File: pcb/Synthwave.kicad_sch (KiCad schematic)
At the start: 61 parts, among them J1 Conn_01x01_Pin, J2 Conn_01x01_Pin, P1 MINI-360, P2 MINI-360, Q1 TIP120, Q10 TIP120, Q2 TIP120, Q3 TIP120, Q4 TIP120, Q5 TIP120, Q6 TIP120, Q7 TIP120, Q8 TIP120, Q9 TIP120, U1 Heltec_HTIT-WB32, U2 L9110

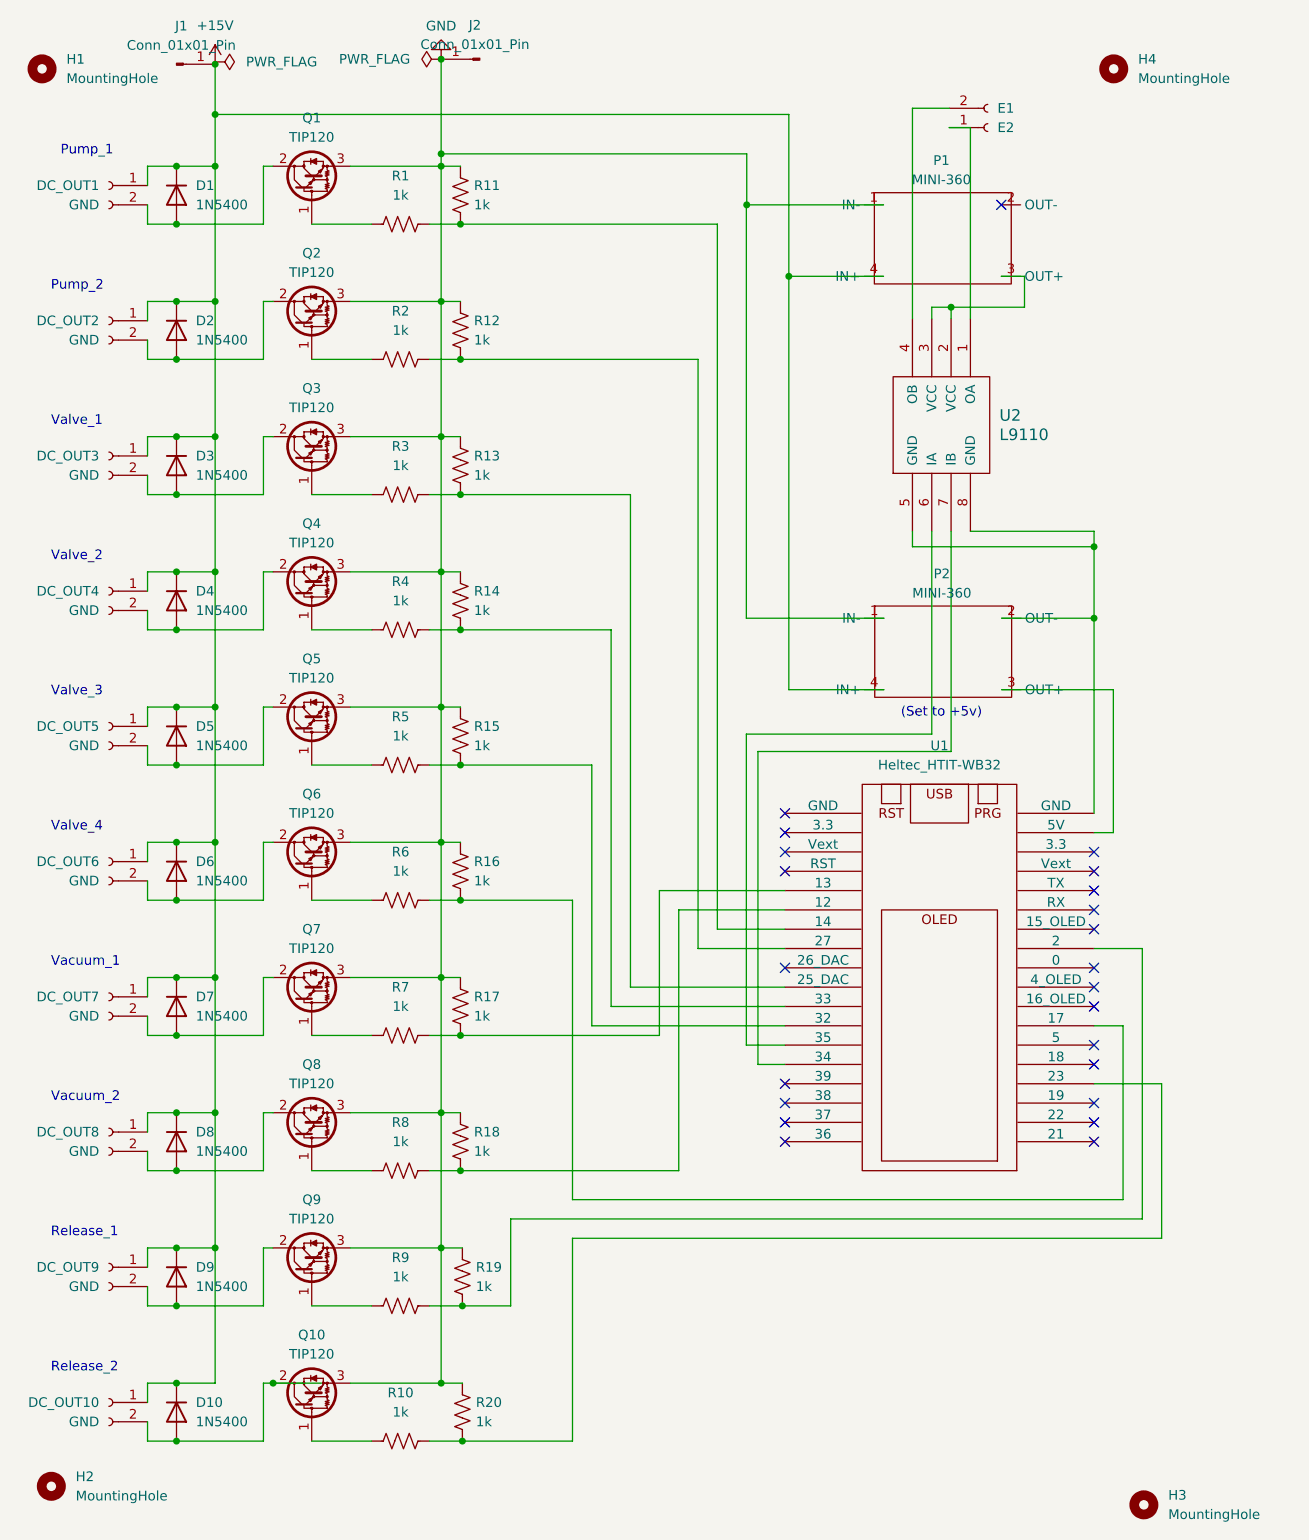
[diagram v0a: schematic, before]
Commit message: Many small updates
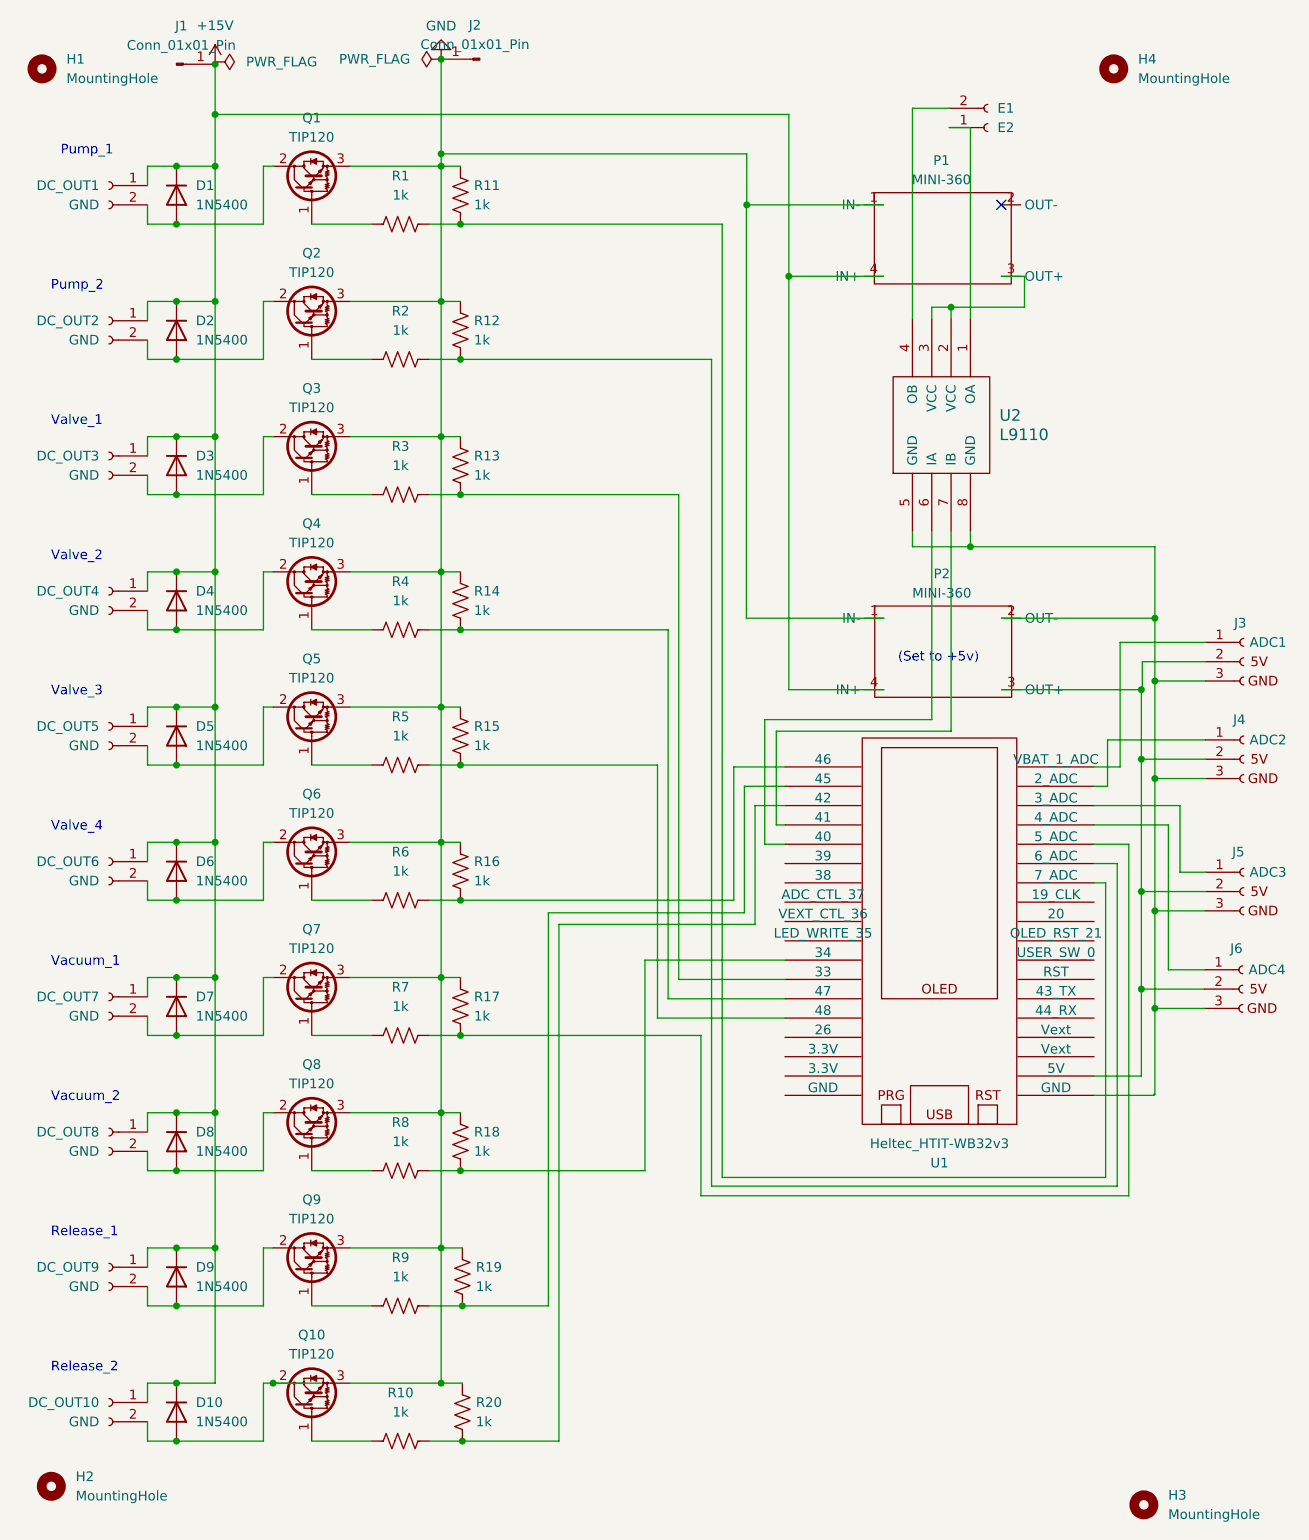
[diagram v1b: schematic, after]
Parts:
- added J3: ADC1, Connector_PinSocket_2.54mm:PinSocket_1x03_P2.54mm_Vertical, symbol Connector:Conn_01x03_Socket
- added J4: ADC2, Connector_PinSocket_2.54mm:PinSocket_1x03_P2.54mm_Vertical, symbol Connector:Conn_01x03_Socket
- added J5: ADC3, Connector_PinSocket_2.54mm:PinSocket_1x03_P2.54mm_Vertical, symbol Connector:Conn_01x03_Socket
- added J6: ADC4, Connector_PinSocket_2.54mm:PinSocket_1x03_P2.54mm_Vertical, symbol Connector:Conn_01x03_Socket
- U1: value Heltec_HTIT-WB32 -> Heltec_HTIT-WB32v3
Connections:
- net at R18.1, R8.2: now also U1.2 (34); no longer U1.12
- net at R16.1, R6.2: now also U1.21 (46); no longer U1.17
- net at R14.1, R4.2: now also U1.3 (47); no longer U1.33
- net at R10.2, R20.1: now also U1.19 (42); no longer U1.23
- net at R1.2, R11.1: now also U1.32 (7_ADC); no longer U1.14
- net at U1.1 (48): now also R15.1, R5.2
- net at R17.1, R7.2: now also U1.34 (5_ADC); no longer U1.13
- net at U1.15 (33): now also R13.1, R3.2
- net at U1.18 (40): now also U2.6 (IA)
- net at R19.1, R9.2: now also U1.22 (45); no longer U1.2
- net at P2.3 (OUT+): now also U1.9 (5V), J3.2 (Pin_2), J4.2 (Pin_2), J5.2 (Pin_2), J6.2 (Pin_2); no longer U1.20 (5V)
- net at R12.1, R2.2: now also U1.35 (6_ADC); no longer U1.27
- net at P2.2 (OUT-), U2.5 (GND), U2.8 (GND): now also U1.8 (GND), J3.3 (PIN_3), J4.3 (PIN_3), J5.3 (PIN_3), J6.3 (PIN_3); no longer U1.28 (GND)
- net at U2.7 (IB): now also U1.23 (41); no longer U1.34
- net at U1.36 (VBAT_1_ADC): now also J3.1 (Pin_1)
- net at U1.37 (2_ADC): now also J4.1 (Pin_1)
- net at U1.38 (3_ADC): now also J5.1 (Pin_1)
- net at U1.39 (4_ADC): now also J6.1 (Pin_1)
- now unconnected: U1.25 (25_DAC)
- no-connect marks 23 -> 1
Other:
- moved on the sheet: U1
